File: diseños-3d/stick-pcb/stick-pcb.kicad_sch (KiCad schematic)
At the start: 34 parts, among them J1 Conn_01x05, J10 Conn_01x02, J11 Conn_01x02, J12 Conn_01x02, J13 Conn_01x02, J14 Conn_01x02, J15 Conn_01x02, J16 Conn_01x02, J17 Conn_01x02, J18 Conn_01x02, J19 Conn_01x02, J2 Conn_01x02, J20 Conn_01x02, J21 Conn_01x02, J22 Conn_01x02, J23 Conn_01x02, J24 Conn_01x02, J25 Conn_01x02, J3 Conn_01x02, J4 Conn_01x02, J5 Conn_01x02, J6 Conn_01x02, J7 Conn_01x02, J8 Conn_01x02, J9 Conn_01x02, U1 4021, U2 4021, U3 4021

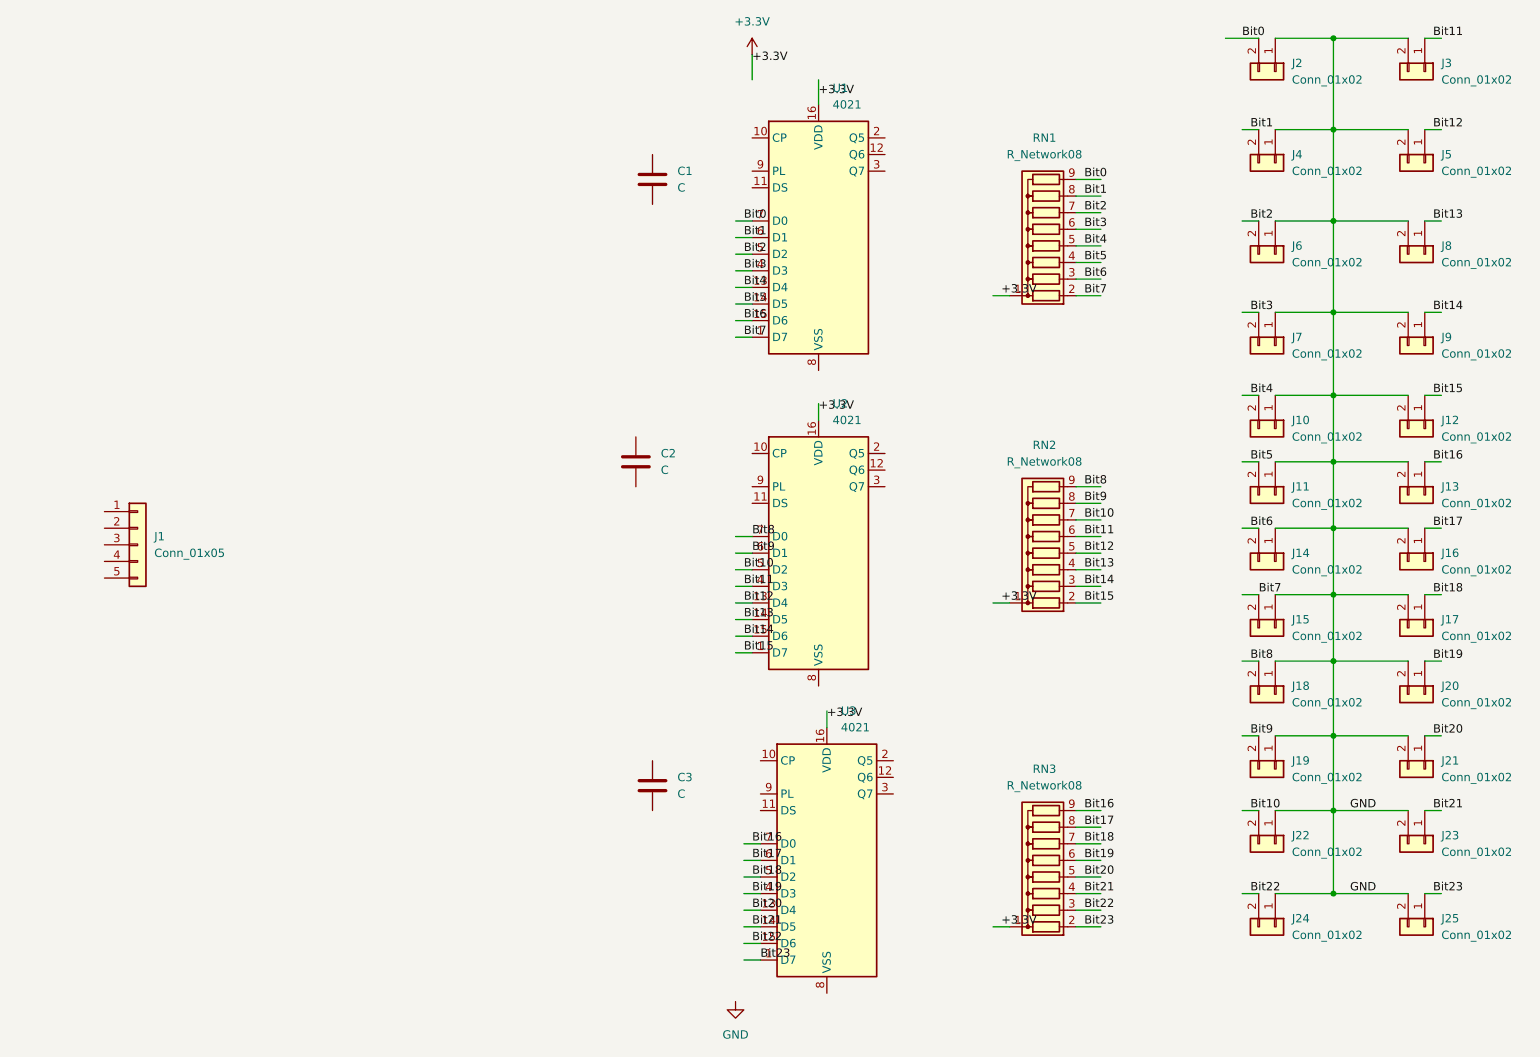
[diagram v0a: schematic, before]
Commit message: terminado el diseño electrónico del grip
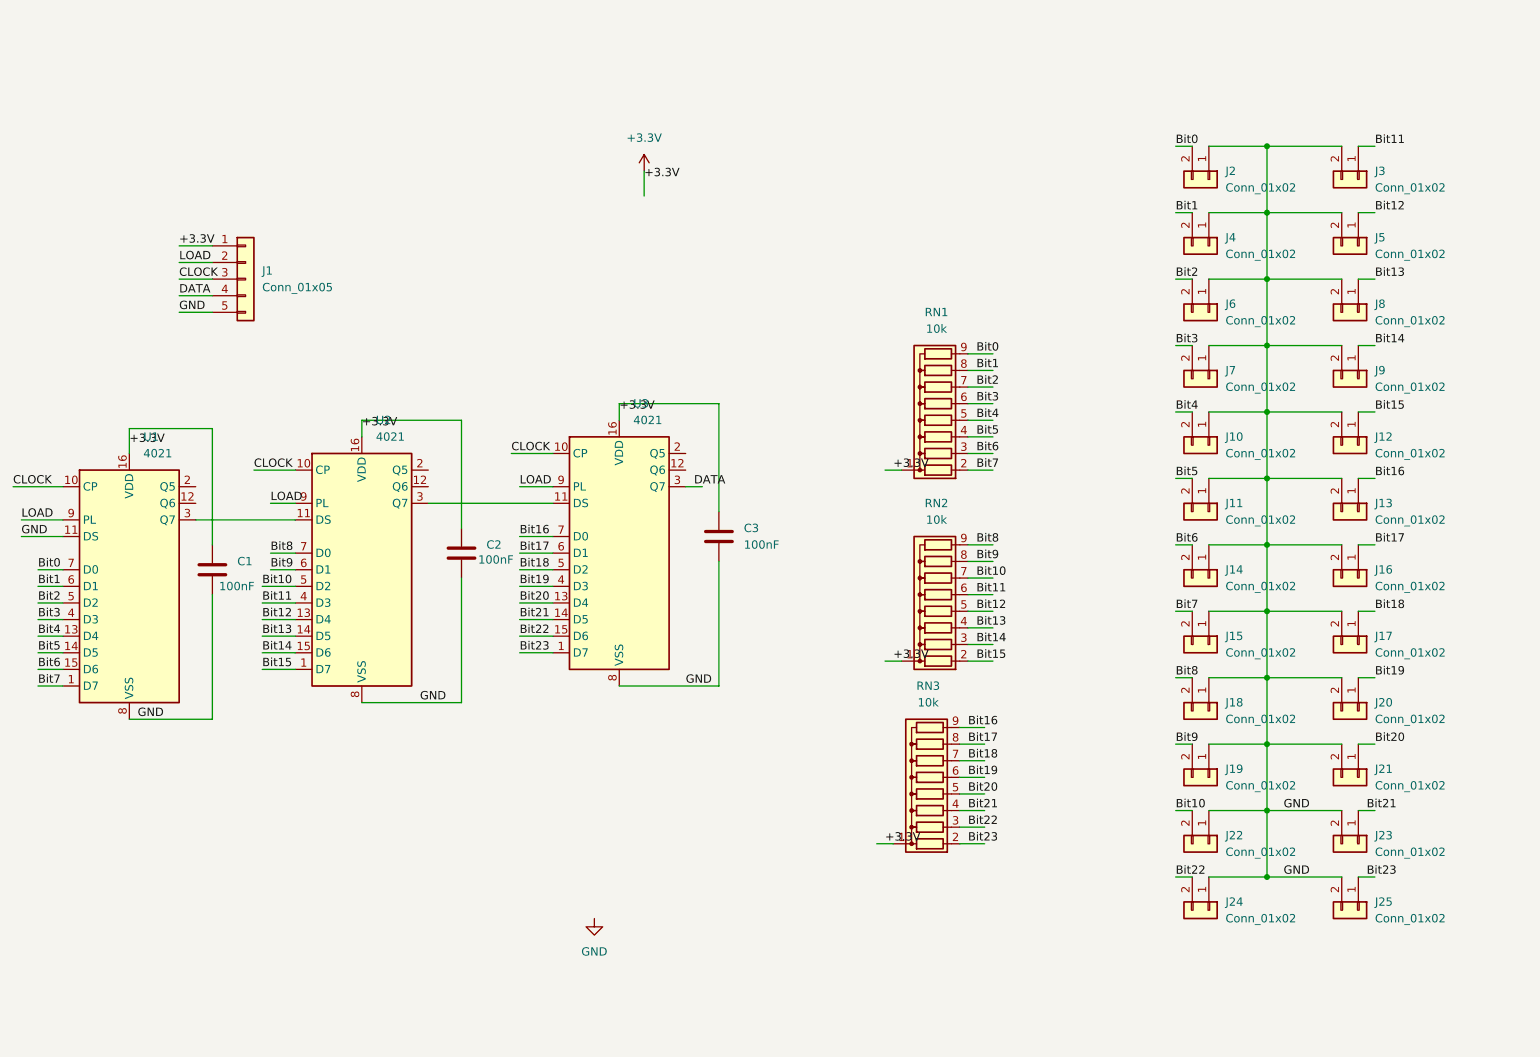
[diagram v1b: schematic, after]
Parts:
- C1, C2, C3: value C -> 100nF
- RN1, RN2, RN3: value R_Network08 -> 10k
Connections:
- net +3.3V: now also C1.1, C2.1, C3.1, J1.1 (Pin_1)
- net GND: now also C1.2, C2.2, C3.2, J1.5 (Pin_5), U1.11 (DS), U1.8 (VSS), U2.8 (VSS), U3.8 (VSS)
- net LOAD: now reaches J1.2 (Pin_2)
- net LOAD: now also U1.9 (PL), U2.9 (PL), U3.9 (PL)
- net CLOCK: now reaches J1.3 (Pin_3)
- net CLOCK: now also U1.10 (CP), U2.10 (CP), U3.10 (CP)
- net DATA: now reaches J1.4 (Pin_4)
- net DATA: now also U3.3 (Q7)
- net at U2.11 (DS): now also U1.3 (Q7)
- net at U2.3 (Q7): now also U3.11 (DS)
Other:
- moved on the sheet: C1, C2, C3, J1, J10, J11, J12, J13, J14, J15, J16, J17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
